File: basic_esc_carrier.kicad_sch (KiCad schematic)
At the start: 9 parts, among them J1 0039301040, J2 0039301040, J3 0039301040, J4 0039301080, J5 0039301080, J6 S4B-PH-K-S

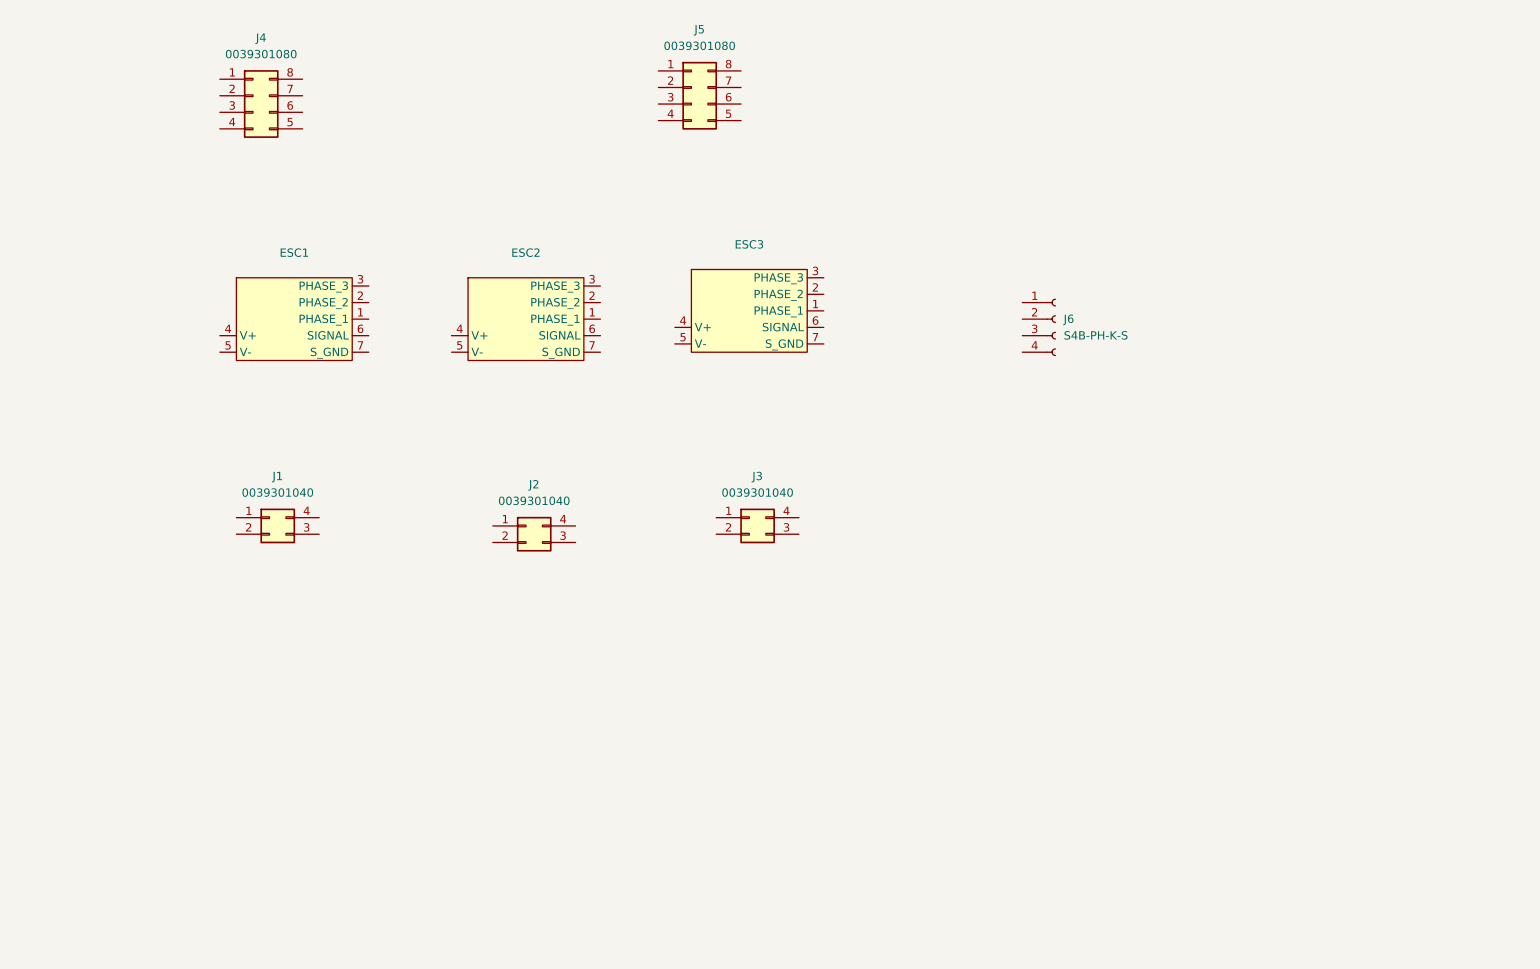
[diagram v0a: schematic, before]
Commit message: finished schematic
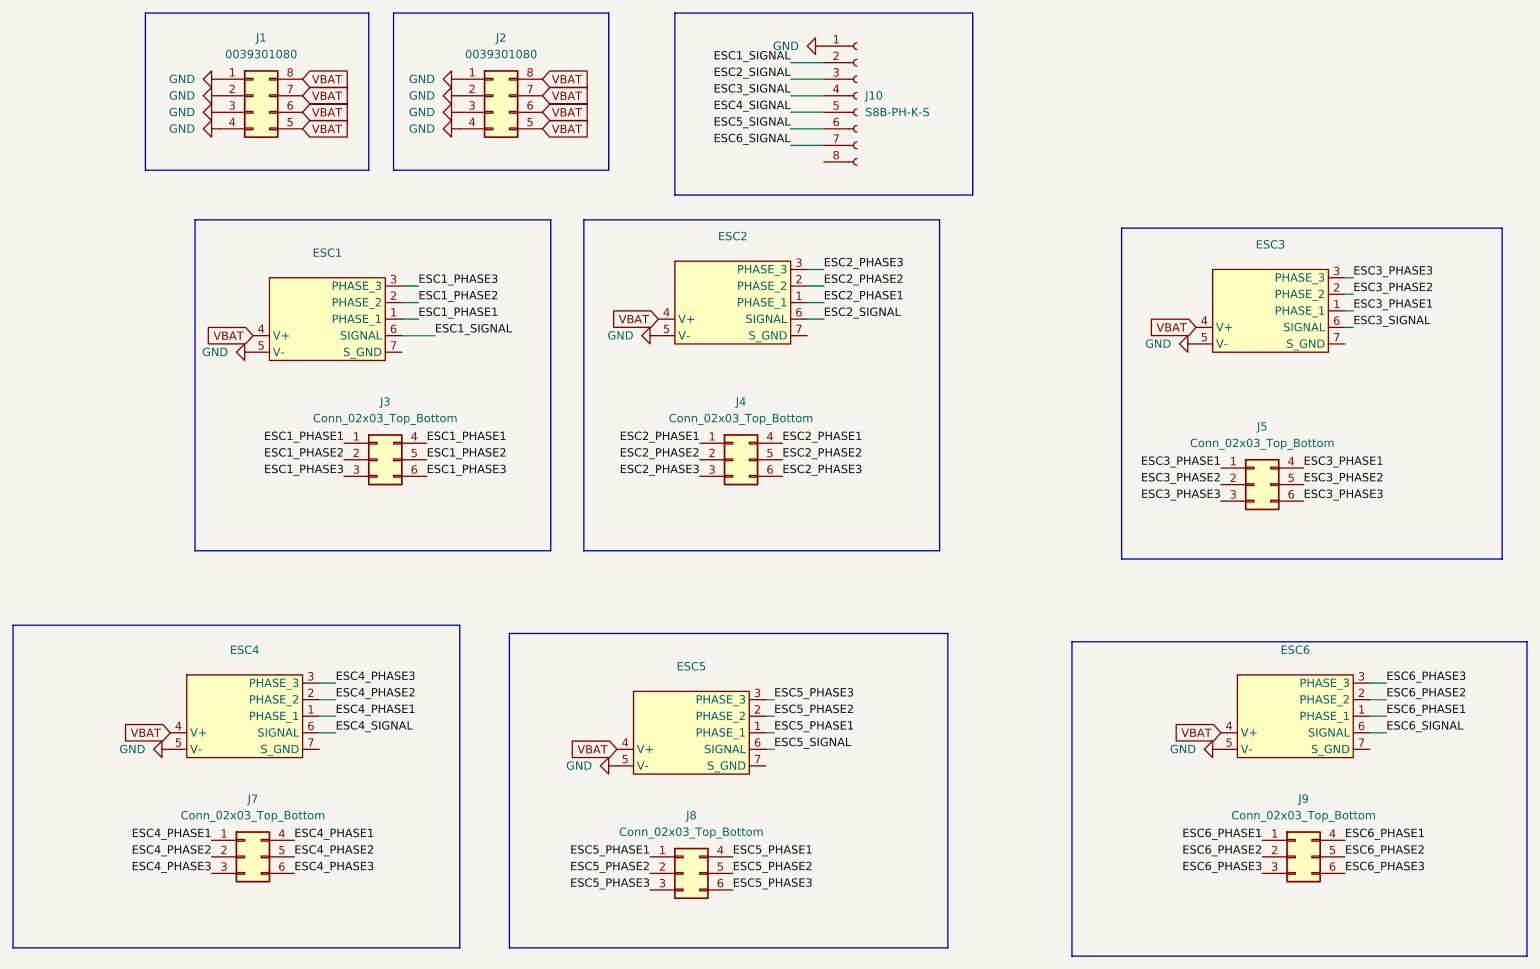
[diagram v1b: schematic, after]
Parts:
- removed J1, J2, J3: 0039301040, Connector_Molex:Molex_Mini-Fit_Jr_5569-04A2_2x02_P4.20mm_Horizontal, symbol Connector_Generic:Conn_02x02_Counter_Clockwise
- removed J5: 0039301080, Connector_Molex:Molex_Mini-Fit_Jr_5569-08A2_2x04_P4.20mm_Horizontal, symbol Connector_Generic:Conn_02x04_Counter_Clockwise
- removed J6: S4B-PH-K-S, Connector_JST:JST_PH_S4B-PH-K_1x04_P2.00mm_Horizontal, symbol Connector:Conn_01x04_Socket
- added ESC4, ESC5, ESC6: ~, basic_esc:basic_esc, symbol basic_esc:Blue_Robotics_Basic_ESC
- added J10: S8B-PH-K-S, Connector_JST:JST_PH_S8B-PH-K_1x08_P2.00mm_Horizontal, symbol Connector:Conn_01x08_Socket
- added J2: 0039301080, Connector_Molex:Molex_Mini-Fit_Jr_5569-08A2_2x04_P4.20mm_Horizontal, symbol Connector_Generic:Conn_02x04_Counter_Clockwise
- added J3, J4, J5, J7, J8, J9: Conn_02x03_Top_Bottom, Connector_Molex:Molex_Mini-Fit_Jr_5569-06A1_2x03_P4.20mm_Horizontal, symbol Connector_Generic:Conn_02x03_Top_Bottom
- ESC1, ESC2, ESC3: footprint (none) -> basic_esc:basic_esc
- renumbered J4 to J1
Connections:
- net ESC1_PHASE1: now reaches ESC1.1 (PHASE_1)
- net ESC1_PHASE1: now also J3.1 (Pin_1), J3.4 (Pin_4)
- net ESC1_PHASE2: now reaches ESC1.2 (PHASE_2)
- net ESC1_PHASE2: now also J3.2 (Pin_2), J3.5 (Pin_5)
- net ESC1_PHASE3: now reaches ESC1.3 (PHASE_3)
- net ESC1_PHASE3: now also J3.3 (Pin_3), J3.6 (Pin_6)
- net VBAT: now reaches ESC1.4 (V+)
- net VBAT: now also ESC2.4 (V+), ESC3.4 (V+), J1.5 (Pin_5), J1.6 (Pin_6), J1.7 (Pin_7), J1.8 (Pin_8), ESC4.4 (V+), ESC5.4 (V+), ESC6.4 (V+), J2.5 (Pin_5), J2.6 (Pin_6), J2.7 (Pin_7), J2.8 (Pin_8)
- net GND: now reaches ESC1.5 (V-)
- net GND: now also ESC2.5 (V-), ESC3.5 (V-), J1.1 (Pin_1), J1.2 (Pin_2), J1.3 (Pin_3), J1.4 (Pin_4), ESC4.5 (V-), ESC5.5 (V-), ESC6.5 (V-), J10.1 (Pin_1), J2.1 (Pin_1), J2.2 (Pin_2), J2.3 (Pin_3), J2.4 (Pin_4)
- net ESC1_SIGNAL: now reaches ESC1.6 (SIGNAL)
- net ESC1_SIGNAL: now also J10.2 (Pin_2)
- net ESC3_PHASE1: now reaches ESC3.1 (PHASE_1)
- net ESC3_PHASE1: now also J5.1 (Pin_1), J5.4 (Pin_4)
- net ESC3_PHASE2: now reaches ESC3.2 (PHASE_2)
- net ESC3_PHASE2: now also J5.2 (Pin_2), J5.5 (Pin_5)
- net ESC3_PHASE3: now reaches ESC3.3 (PHASE_3)
- net ESC3_PHASE3: now also J5.3 (Pin_3), J5.6 (Pin_6)
- net ESC3_SIGNAL: now reaches ESC3.6 (SIGNAL)
- net ESC3_SIGNAL: now also J10.4 (Pin_4)
- net ESC2_PHASE1: now reaches ESC2.1 (PHASE_1)
- net ESC2_PHASE1: now also J4.1 (Pin_1), J4.4 (Pin_4)
- net ESC2_PHASE2: now reaches ESC2.2 (PHASE_2)
- net ESC2_PHASE2: now also J4.2 (Pin_2), J4.5 (Pin_5)
- net ESC2_PHASE3: now reaches ESC2.3 (PHASE_3)
- net ESC2_PHASE3: now also J4.3 (Pin_3), J4.6 (Pin_6)
- net ESC2_SIGNAL: now reaches ESC2.6 (SIGNAL)
- net ESC2_SIGNAL: now also J10.3 (Pin_3)
- new net ESC4_PHASE1: ESC4.1 (PHASE_1), J7.1 (Pin_1), J7.4 (Pin_4)
- new net ESC4_PHASE2: ESC4.2 (PHASE_2), J7.2 (Pin_2), J7.5 (Pin_5)
- new net ESC4_PHASE3: ESC4.3 (PHASE_3), J7.3 (Pin_3), J7.6 (Pin_6)
- new net ESC4_SIGNAL: ESC4.6 (SIGNAL), J10.5 (Pin_5)
- new net ESC5_PHASE1: ESC5.1 (PHASE_1), J8.1 (Pin_1), J8.4 (Pin_4)
- new net ESC5_PHASE2: ESC5.2 (PHASE_2), J8.2 (Pin_2), J8.5 (Pin_5)
- new net ESC5_PHASE3: ESC5.3 (PHASE_3), J8.3 (Pin_3), J8.6 (Pin_6)
- new net ESC5_SIGNAL: ESC5.6 (SIGNAL), J10.6 (Pin_6)
- new net ESC6_PHASE1: ESC6.1 (PHASE_1), J9.1 (Pin_1), J9.4 (Pin_4)
- new net ESC6_PHASE2: ESC6.2 (PHASE_2), J9.2 (Pin_2), J9.5 (Pin_5)
- new net ESC6_PHASE3: ESC6.3 (PHASE_3), J9.3 (Pin_3), J9.6 (Pin_6)
- new net ESC6_SIGNAL: ESC6.6 (SIGNAL), J10.7 (Pin_7)
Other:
- moved on the sheet: ESC1, ESC2, ESC3
